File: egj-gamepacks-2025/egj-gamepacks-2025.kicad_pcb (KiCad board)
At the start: 2 copper layers, 52.3 x 64 mm, 84 parts, among them J1 USB_B_Micro, J3 SM03B-SRSS-TB, J5 GameBoy_GamePak_AGB-002, SW1 SW_Push, SW2 SW_Push, U1 W25Q128JVS, U10 SP3012-06UTG, U11 VL6180XV0NR_1, U12 TXS0108EPW, U13 LD1117S18TR_SOT223, U14 BNO055, U2 DNF, U3 NCP1117-3.3_SOT223, U4 RP2350_80QFN, U5 USBLC6-2P6, U6 SP3012-06UTG, U7 SP3012-06UTG, U8 SP3012-06UTG, U9 SP3012-06UTG, Y1 ABM8-272-T3

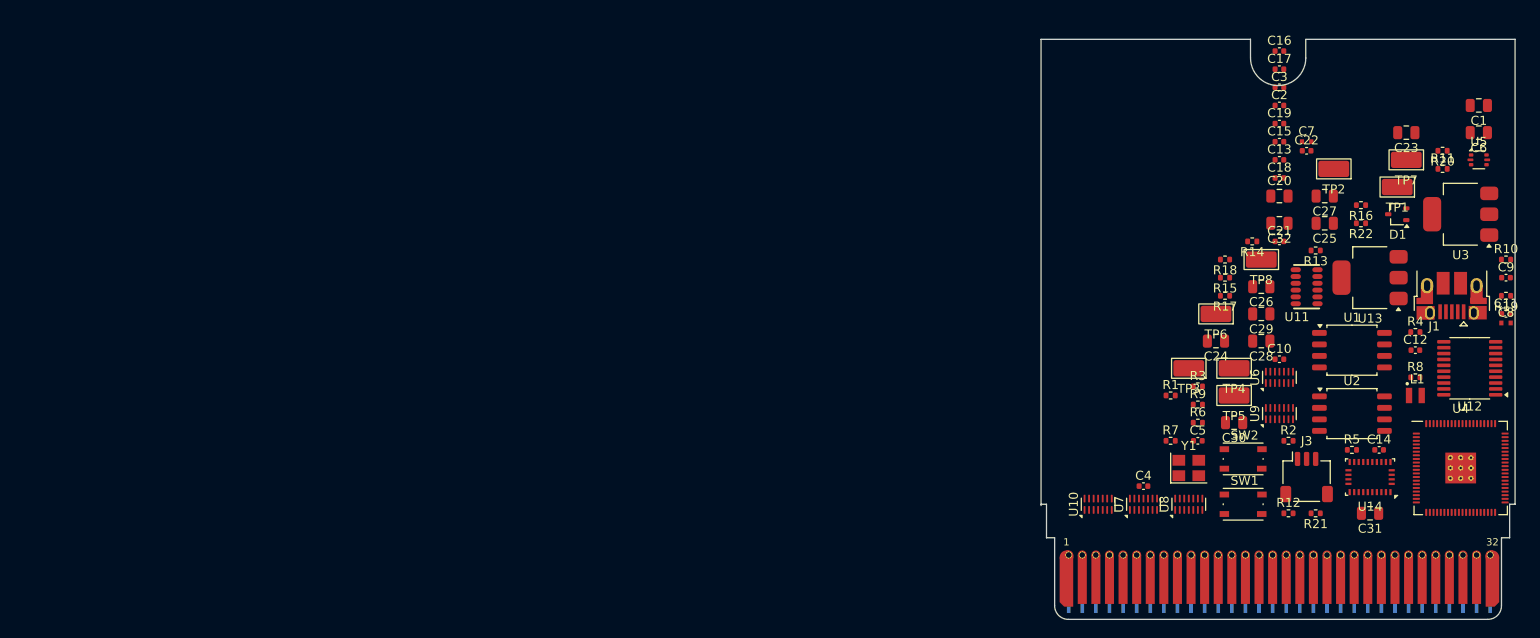
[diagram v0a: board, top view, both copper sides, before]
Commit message: Update
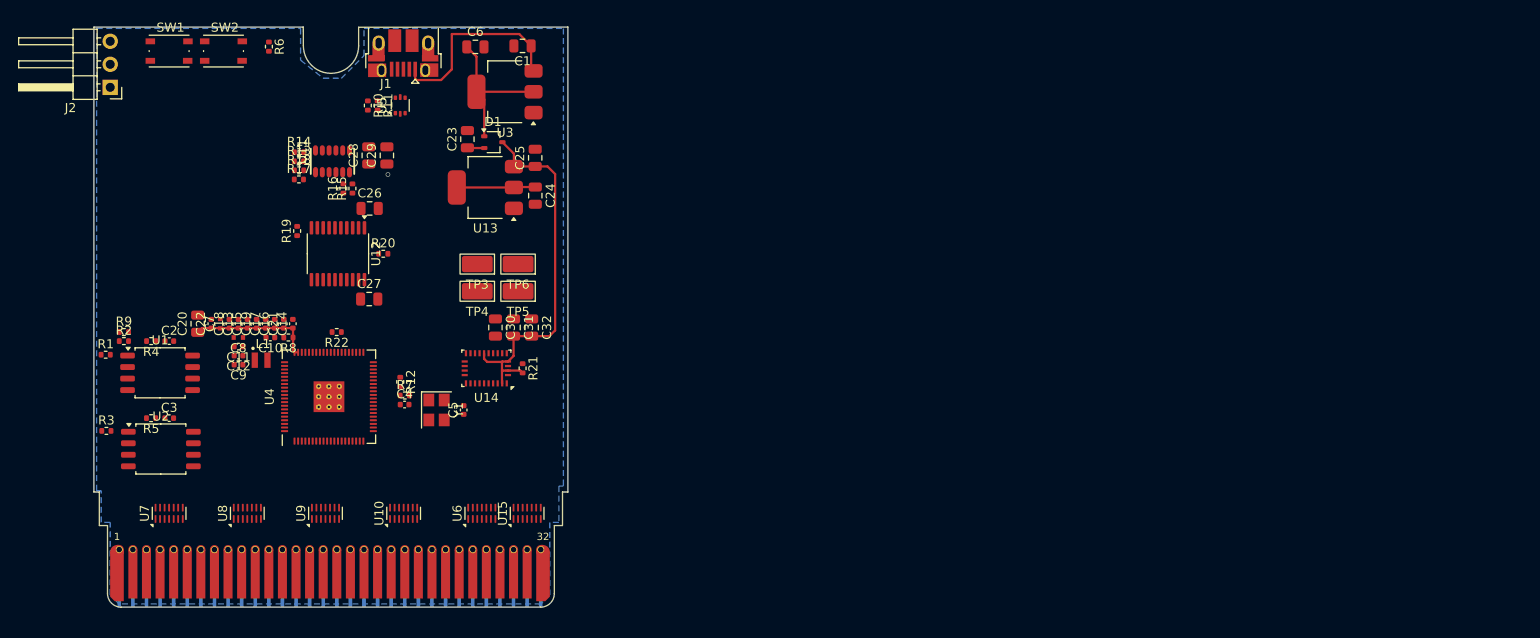
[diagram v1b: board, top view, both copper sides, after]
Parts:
- removed J3: SM03B-SRSS-TB, Connector_JST:JST_SH_SM03B-SRSS-TB_1x03-1MP_P1.00mm_Horizontal
- removed TP1, TP2, TP7, TP8: TestPoint, TestPoint:TestPoint_Keystone_5015_Micro_Mini
- added J2: Conn_01x03_Pin, Connector_PinHeader_2.54mm:PinHeader_1x03_P2.54mm_Horizontal, F.Cu at (119.0, 66.0)
- added U15: SP3012-06UTG, Package_DFN_QFN:DFN-14_1.35x3.5mm_P0.5mm, F.Cu at (165.0, 113.0)
- moved C9 140.2 mm to (133.2, 96.6), turned to 180 degrees
- moved C11 139.9 mm to (133.2, 94.6), turned to 180 degrees
- moved C8 139.9 mm to (133.1, 93.6), turned to 180 degrees
- moved R4 139.5 mm to (123.5, 94.0), turned to 180 degrees
- moved R19 133.6 mm to (139.6, 81.9), turned to 90 degrees
- moved R5 132.5 mm to (123.5, 102.5), turned to 180 degrees
- moved U1 131.5 mm to (124.5, 97.5)
- moved U2 131.5 mm to (124.6, 105.9)
- moved C12 129.8 mm to (133.2, 95.6), turned to 180 degrees
- moved R2 129.0 mm to (120.5, 94.0)
- moved SW1 128.6 mm to (125.5, 62.0)
- moved C3 127.8 mm to (125.5, 102.5)
- moved L1 127.4 mm to (135.7, 96.1)
- moved R10 126.7 mm to (147.4, 68.0), turned to -90 degrees
- moved U12 125.5 mm to (144.1, 84.4), turned to -90 degrees
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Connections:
- net +1V1 renamed /RP2350/+1V1
- D1 pad 1: +3V3_GBA -> +3V3_USB
- D1 pad 2: +3V3_USB -> +3V3_GBA
- R10 pad 1: /RP2350/USB_D+ -> /Power/USB.USB_D_C+
- R11 pad 1: /RP2350/USB_D- -> /Power/USB.USB_D_C-
- U10 pad 1: unconnected-(U10-Pad1) -> /GBA_Connector/GBA_ADD13
- U10 pad 11: /GBA_Connector/GBA_SIG.N_CS -> /GBA_Connector/GBA_DATA0
- U10 pad 12: /GBA_Connector/GBA_SIG.N_RD -> /GBA_Connector/GBA_ADD15
- U10 pad 13: /GBA_Connector/GBA_SIG.N_WR -> /GBA_Connector/GBA_ADD14
- U10 pad 14: /GBA_Connector/GBA_SIG.PHI -> /GBA_Connector/GBA_ADD13
- U10 pad 2: unconnected-(U10-Pad2) -> /GBA_Connector/GBA_ADD14
- U10 pad 3: unconnected-(U10-Pad3) -> /GBA_Connector/GBA_ADD15
- U10 pad 4: unconnected-(U10-Pad4) -> /GBA_Connector/GBA_DATA0
- U10 pad 5: unconnected-(U10-Pad5) -> GND
- U10 pad 6: unconnected-(U10-Pad6) -> /GBA_Connector/GBA_DATA1
- U10 pad 7: unconnected-(U10-Pad7) -> /GBA_Connector/GBA_DATA2
- U10 pad 8: /GBA_Connector/GBA_SIG.IRQ -> /GBA_Connector/GBA_DATA2
- U10 pad 9: /GBA_Connector/GBA_SIG.N_CS2 -> /GBA_Connector/GBA_DATA1
- U4 pad 1: /GBA_Connector/GBA_DATA4 -> /GBA_Connector/GBA_ADD0
- U4 pad 11: /GBA_Connector/GBA_ADD4 -> /GBA_Connector/GBA_ADD8
- U4 pad 12: /GBA_Connector/GBA_ADD5 -> /GBA_Connector/GBA_ADD9
- U4 pad 13: /GBA_Connector/GBA_ADD6 -> /GBA_Connector/GBA_ADD10
- U4 pad 14: /GBA_Connector/GBA_ADD7 -> /GBA_Connector/GBA_ADD11
- U4 pad 16: /GBA_Connector/GBA_ADD8 -> /GBA_Connector/GBA_ADD12
- U4 pad 17: /GBA_Connector/GBA_ADD9 -> /GBA_Connector/GBA_ADD13
- U4 pad 18: /GBA_Connector/GBA_ADD10 -> /GBA_Connector/GBA_ADD14
- U4 pad 19: /GBA_Connector/GBA_ADD11 -> /GBA_Connector/GBA_ADD15
- U4 pad 2: /GBA_Connector/GBA_DATA5 -> /GBA_Connector/GBA_ADD1
- U4 pad 20: /GBA_Connector/GBA_ADD12 -> /GBA_Connector/GBA_DATA0
- U4 pad 21: /GBA_Connector/GBA_ADD13 -> /GBA_Connector/GBA_DATA1
- U4 pad 22: /GBA_Connector/GBA_ADD14 -> /GBA_Connector/GBA_DATA2
- U4 pad 23: /GBA_Connector/GBA_ADD15 -> /GBA_Connector/GBA_DATA3
- U4 pad 25: /GBA_Connector/GBA_SIG.PHI -> /GBA_Connector/GBA_DATA4
- U4 pad 26: /GBA_Connector/GBA_SIG.N_WR -> /GBA_Connector/GBA_DATA5
- U4 pad 27: /GBA_Connector/GBA_SIG.N_RD -> /GBA_Connector/GBA_DATA6
- U4 pad 28: /GBA_Connector/GBA_SIG.N_CS -> /GBA_Connector/GBA_DATA7
- U4 pad 3: /GBA_Connector/GBA_DATA6 -> /GBA_Connector/GBA_ADD2
- U4 pad 4: /GBA_Connector/GBA_DATA7 -> /GBA_Connector/GBA_ADD3
- U4 pad 6: /GBA_Connector/GBA_ADD0 -> /GBA_Connector/GBA_ADD4
- U4 pad 7: /GBA_Connector/GBA_ADD1 -> /GBA_Connector/GBA_ADD5
- U4 pad 77: /GBA_Connector/GBA_DATA0 -> /GBA_Connector/GBA_SIG.PHI
- U4 pad 78: /GBA_Connector/GBA_DATA1 -> /GBA_Connector/GBA_SIG.N_WR
- U4 pad 79: /GBA_Connector/GBA_DATA2 -> /GBA_Connector/GBA_SIG.N_RD
- U4 pad 8: /GBA_Connector/GBA_ADD2 -> /GBA_Connector/GBA_ADD6
- U4 pad 80: /GBA_Connector/GBA_DATA3 -> /GBA_Connector/GBA_SIG.N_CS
- U4 pad 9: /GBA_Connector/GBA_ADD3 -> /GBA_Connector/GBA_ADD7
- U5 pad 2: GND -> unconnected-(U5-GND-Pad2)
- U5 pad 4: /RP2350/USB_D- -> /Power/USB.USB_D_C-
- U5 pad 5: unconnected-(U5-VBUS-Pad5) -> GND
- U5 pad 6: /RP2350/USB_D+ -> /Power/USB.USB_D_C+
- U6 pad 1: unconnected-(U6-Pad1) -> /GBA_Connector/GBA_DATA3
- U6 pad 11: /GBA_Connector/GBA_DATA3 -> /GBA_Connector/GBA_DATA6
- U6 pad 12: /GBA_Connector/GBA_DATA2 -> /GBA_Connector/GBA_DATA5
- U6 pad 13: /GBA_Connector/GBA_DATA1 -> /GBA_Connector/GBA_DATA4
- U6 pad 14: /GBA_Connector/GBA_DATA0 -> /GBA_Connector/GBA_DATA3
- U6 pad 2: unconnected-(U6-Pad2) -> /GBA_Connector/GBA_DATA4
- U6 pad 3: unconnected-(U6-Pad3) -> /GBA_Connector/GBA_DATA5
- U6 pad 4: unconnected-(U6-Pad4) -> /GBA_Connector/GBA_DATA6
- U6 pad 5: unconnected-(U6-Pad5) -> GND
- U6 pad 6: unconnected-(U6-Pad6) -> /GBA_Connector/GBA_DATA7
- U6 pad 7: unconnected-(U6-Pad7) -> /GBA_Connector/GBA_SIG.N_CS2
- U6 pad 8: /GBA_Connector/GBA_DATA5 -> /GBA_Connector/GBA_SIG.N_CS2
- U6 pad 9: /GBA_Connector/GBA_DATA4 -> /GBA_Connector/GBA_DATA7
- U7 pad 1: unconnected-(U7-Pad1) -> /GBA_Connector/GBA_SIG.PHI
- U7 pad 11: /GBA_Connector/GBA_ADD1 -> /GBA_Connector/GBA_SIG.N_CS
- U7 pad 12: /GBA_Connector/GBA_ADD0 -> /GBA_Connector/GBA_SIG.N_RD
- U7 pad 13: /GBA_Connector/GBA_DATA7 -> /GBA_Connector/GBA_SIG.N_WR
- U7 pad 14: /GBA_Connector/GBA_DATA6 -> /GBA_Connector/GBA_SIG.PHI
- U7 pad 2: unconnected-(U7-Pad2) -> /GBA_Connector/GBA_SIG.N_WR
- U7 pad 3: unconnected-(U7-Pad3) -> /GBA_Connector/GBA_SIG.N_RD
- U7 pad 4: unconnected-(U7-Pad4) -> /GBA_Connector/GBA_SIG.N_CS
- U7 pad 5: unconnected-(U7-Pad5) -> GND
- U7 pad 6: unconnected-(U7-Pad6) -> /GBA_Connector/GBA_ADD0
- U7 pad 7: unconnected-(U7-Pad7) -> /GBA_Connector/GBA_ADD1
- U7 pad 8: /GBA_Connector/GBA_ADD3 -> /GBA_Connector/GBA_ADD1
- U7 pad 9: /GBA_Connector/GBA_ADD2 -> /GBA_Connector/GBA_ADD0
- U8 pad 1: unconnected-(U8-Pad1) -> /GBA_Connector/GBA_ADD2
- U8 pad 11: /GBA_Connector/GBA_ADD7 -> /GBA_Connector/GBA_ADD4
- U8 pad 12: /GBA_Connector/GBA_ADD6 -> /GBA_Connector/GBA_ADD3
- U8 pad 13: /GBA_Connector/GBA_ADD5 -> /GBA_Connector/GBA_ADD2
- U8 pad 14: /GBA_Connector/GBA_ADD4 -> /GBA_Connector/GBA_ADD2
- U8 pad 2: unconnected-(U8-Pad2) -> /GBA_Connector/GBA_ADD2
- U8 pad 3: unconnected-(U8-Pad3) -> /GBA_Connector/GBA_ADD3
- U8 pad 4: unconnected-(U8-Pad4) -> /GBA_Connector/GBA_ADD4
- U8 pad 5: unconnected-(U8-Pad5) -> GND
- U8 pad 6: unconnected-(U8-Pad6) -> /GBA_Connector/GBA_ADD5
- U8 pad 7: unconnected-(U8-Pad7) -> /GBA_Connector/GBA_ADD6
- U8 pad 8: /GBA_Connector/GBA_ADD9 -> /GBA_Connector/GBA_ADD6
- U8 pad 9: /GBA_Connector/GBA_ADD8 -> /GBA_Connector/GBA_ADD5
- U9 pad 1: unconnected-(U9-Pad1) -> /GBA_Connector/GBA_ADD7
- U9 pad 11: /GBA_Connector/GBA_ADD13 -> /GBA_Connector/GBA_ADD10
- U9 pad 12: /GBA_Connector/GBA_ADD12 -> /GBA_Connector/GBA_ADD9
- U9 pad 13: /GBA_Connector/GBA_ADD11 -> /GBA_Connector/GBA_ADD8
- U9 pad 14: /GBA_Connector/GBA_ADD10 -> /GBA_Connector/GBA_ADD7
- U9 pad 2: unconnected-(U9-Pad2) -> /GBA_Connector/GBA_ADD8
- U9 pad 3: unconnected-(U9-Pad3) -> /GBA_Connector/GBA_ADD9
- U9 pad 4: unconnected-(U9-Pad4) -> /GBA_Connector/GBA_ADD10
- U9 pad 5: unconnected-(U9-Pad5) -> GND
- U9 pad 6: unconnected-(U9-Pad6) -> /GBA_Connector/GBA_ADD11
- U9 pad 7: unconnected-(U9-Pad7) -> /GBA_Connector/GBA_ADD12
- U9 pad 8: /GBA_Connector/GBA_ADD15 -> /GBA_Connector/GBA_ADD12
- U9 pad 9: /GBA_Connector/GBA_ADD14 -> /GBA_Connector/GBA_ADD11
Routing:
- net +3V3: track 0.00 -> 55.3 mm
- net VBUS: track 0.00 -> 21.7 mm
- net +3V3_USB: track 0.00 -> 17.0 mm
- net +1V8: track 0.00 -> 8.68 mm
- net +3V3_GBA: track 0.00 -> 1.87 mm
- net (no net): vias 0 -> 1
- added copper zone on B.Cu, net (none)
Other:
- outline, holes or cut-outs redrawn
